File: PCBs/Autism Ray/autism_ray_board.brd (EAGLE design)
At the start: 100 x 80 mm, 6 parts, among them U1 RFM95W-915S2, U2 RASPBERRY_PICOSMD

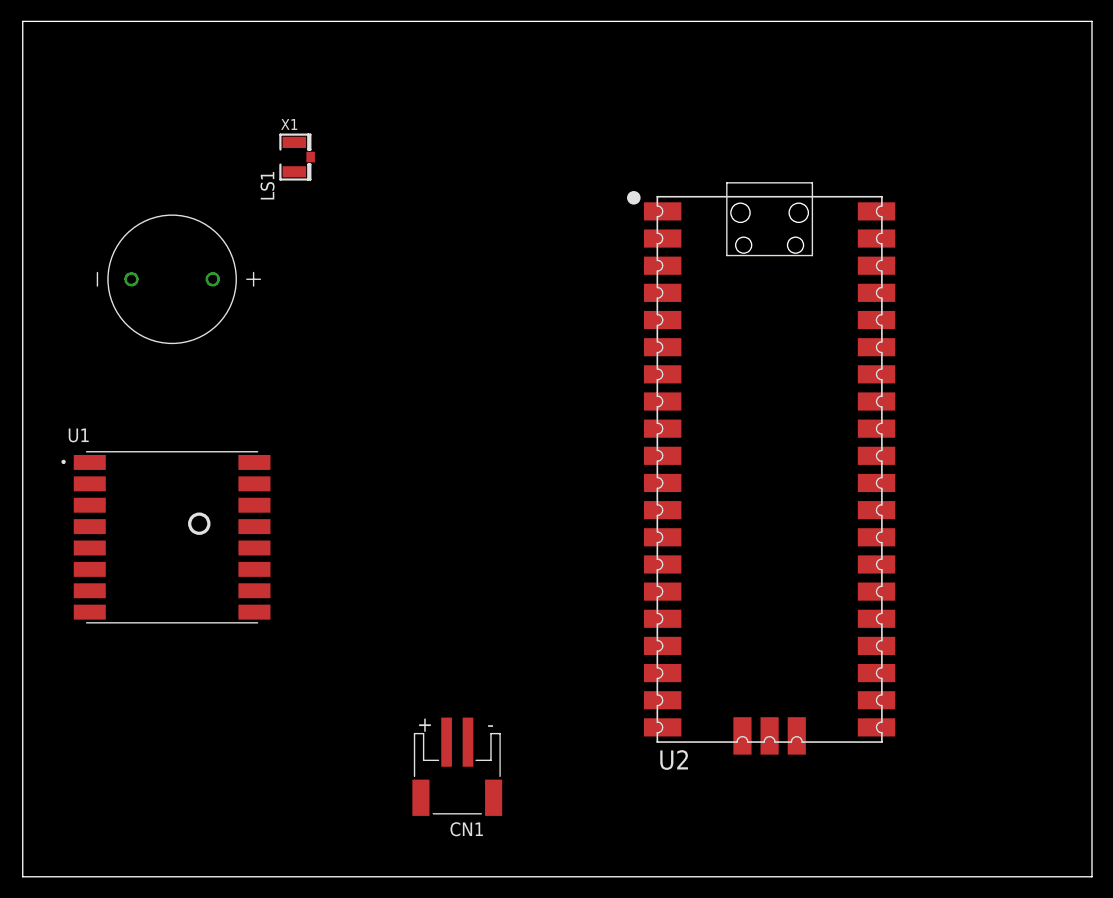
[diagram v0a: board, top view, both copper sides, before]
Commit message: Update PCB
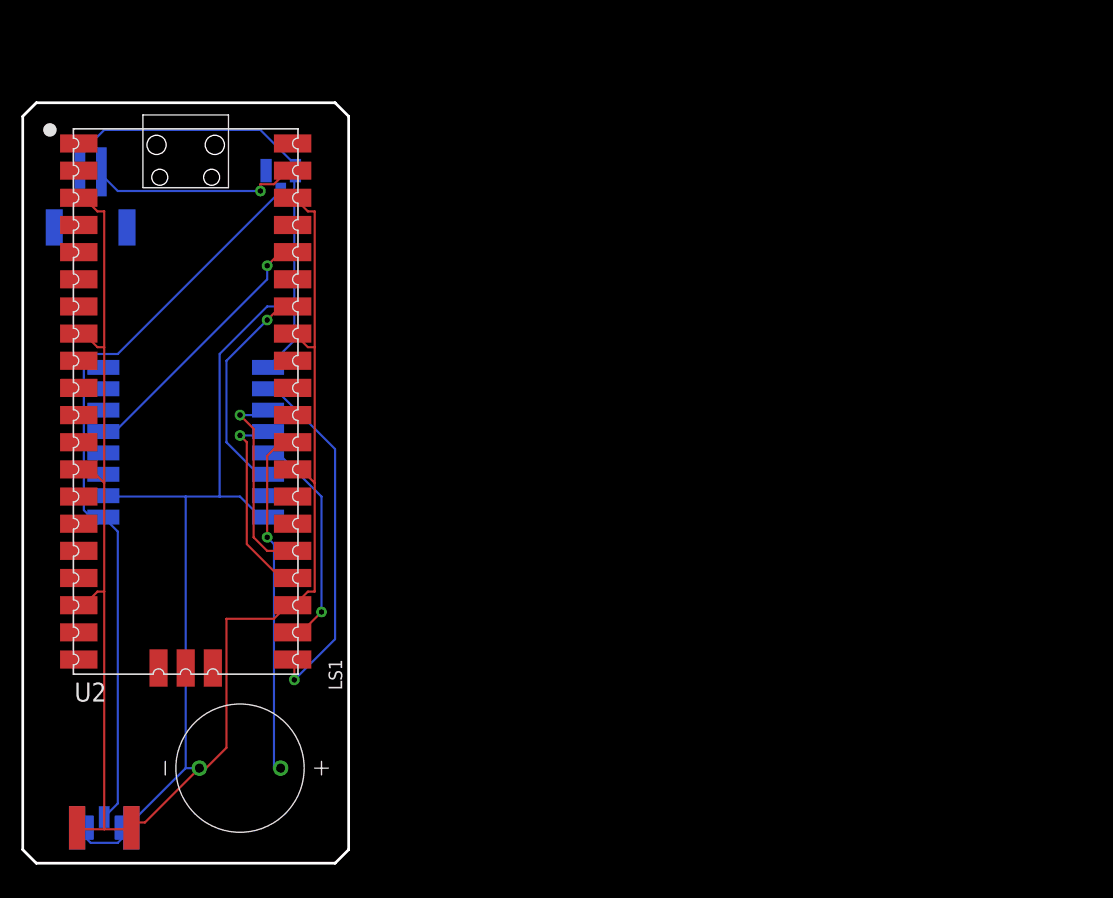
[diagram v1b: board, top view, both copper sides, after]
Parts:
- removed U$1: (no value), microbuilder:PCBFEAT-REV-040
- added X2: (no value), adafruit:SMA_EDGELAUNCH_UFL
- moved CN1 63.4 mm to (6.35, 62.2), flipped to the bottom
- moved U2 55.0 mm to (15.2, 44.5)
- moved LS1 46.2 mm to (20.3, 10.2)
- moved U1 8.98 mm to (15.2, 40.6), flipped to the bottom
- moved X1 1.80 mm to (24.1, 66.0), flipped to the bottom, turned to 270 degrees
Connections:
- net ANT: now also X2.P
- net GND: now also X2.GND@1, X2.GND@2, X2.GND@3, X2.GND@4
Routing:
- net GND: track 0.00 -> 275.9 mm
- net ANT: track 0.00 -> 71.5 mm
- net MISO: track 0.00 -> 33.8 mm, vias 0 -> 1
- net BEEP: track 0.00 -> 33.0 mm, vias 0 -> 1
- net 3.3V: track 0.00 -> 25.5 mm, vias 0 -> 1
- net RST: track 0.00 -> 21.2 mm, vias 0 -> 1
- net CS: track 0.00 -> 20.9 mm, vias 0 -> 1
- net VCC: track 0.00 -> 19.9 mm, vias 0 -> 1
- net MOSI: track 0.00 -> 19.1 mm, vias 0 -> 1
- net SCK: track 0.00 -> 18.9 mm, vias 0 -> 1
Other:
- board size 100 x 80 mm -> 30.5 x 71.1 mm
